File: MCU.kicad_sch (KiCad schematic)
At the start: 28 parts, among them J5 Conn_01x12, Q5 MMBT3904, Q6 MMBT3904, SW1 SW_DPDT_x2, SW2 PTS647SN50SMTR2_LFS, SW3 PTS647SN50SMTR2_LFS, U4 CP2102N-Axx-xQFN28, U5 ESP32-C3-WROOM-02, U6 LIS3DH

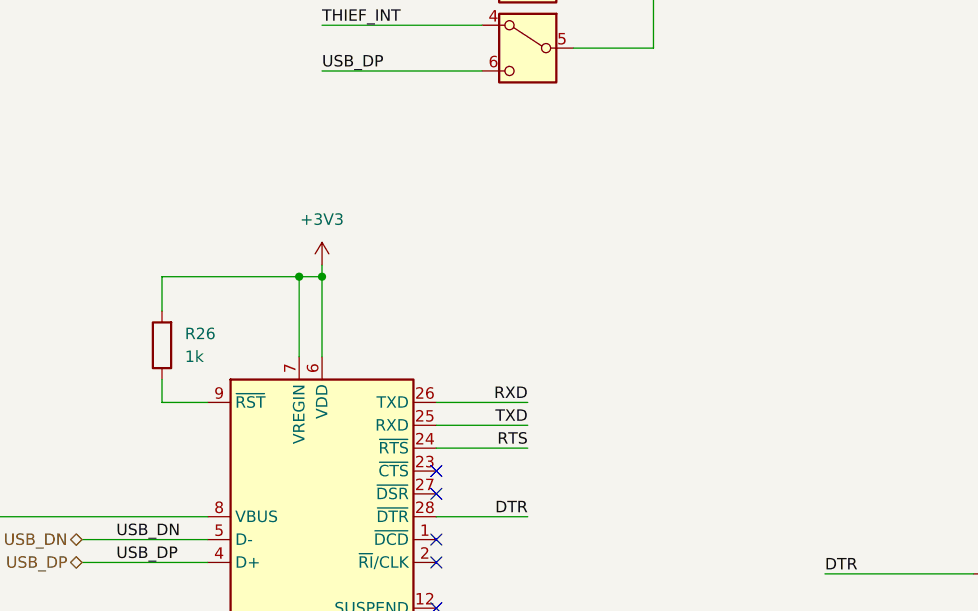
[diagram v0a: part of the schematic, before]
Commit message: first pass layout
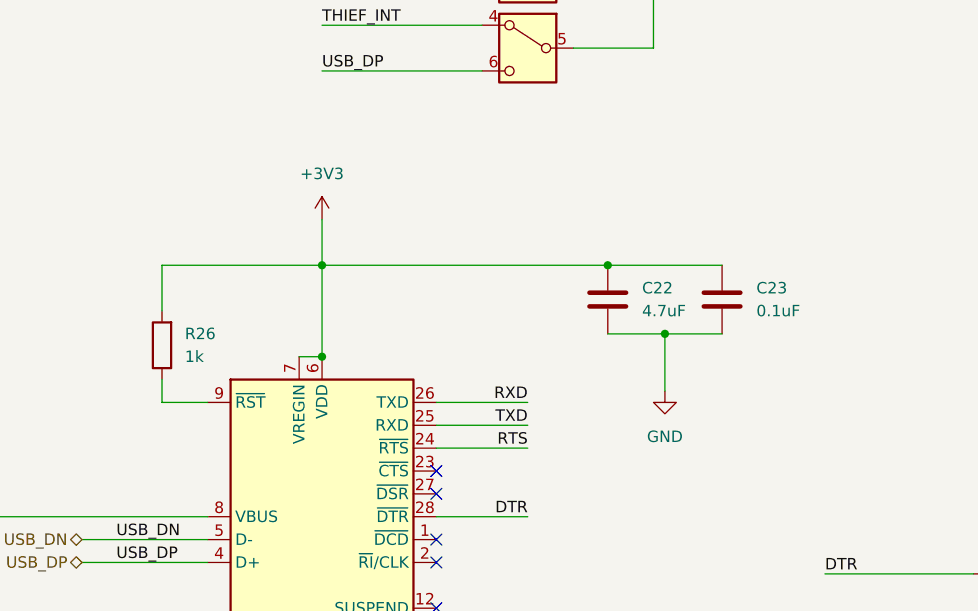
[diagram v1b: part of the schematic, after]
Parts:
- added C22: 4.7uF, Capacitor_SMD:C_0603_1608Metric, symbol Device:C
- added C23: 0.1uF, Capacitor_SMD:C_0603_1608Metric, symbol Device:C
- U5: footprint RF_Module:ESP32-C3-WROOM-02 -> custom_footprints:ESP32-C3-WROOM
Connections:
- net +3V3: now also C22.1, C23.1
- net GND: now also C22.2, C23.2
